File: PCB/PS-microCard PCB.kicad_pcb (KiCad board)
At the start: 4 copper layers, 36.2 x 87.7 mm, 69 parts, among them J1 Oled Socket, J3 MEM2052-00-195-00-A_REVA, J4 10118194-0001LF, J6 JST Debug Connector, SW1 FSM4JSMA, SW2 FSM4JSMA, U1 W25Q128JVS, U2 RP2350_60QFN, U3 TPS2113APWR, U4 TLV75533PDBVR, U5 TPS7A2033PDBVR, Y1 ABM8-272-T3

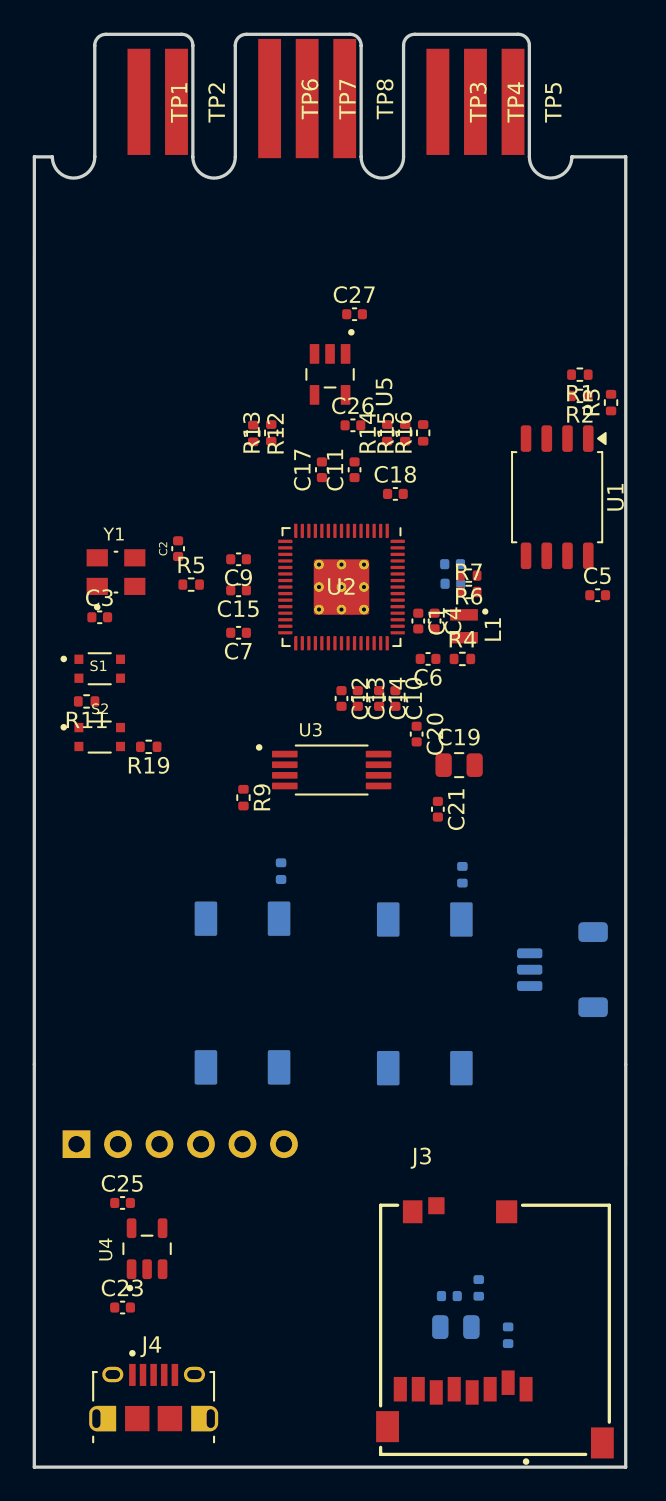
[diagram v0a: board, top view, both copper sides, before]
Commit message: BOM and Gerber files
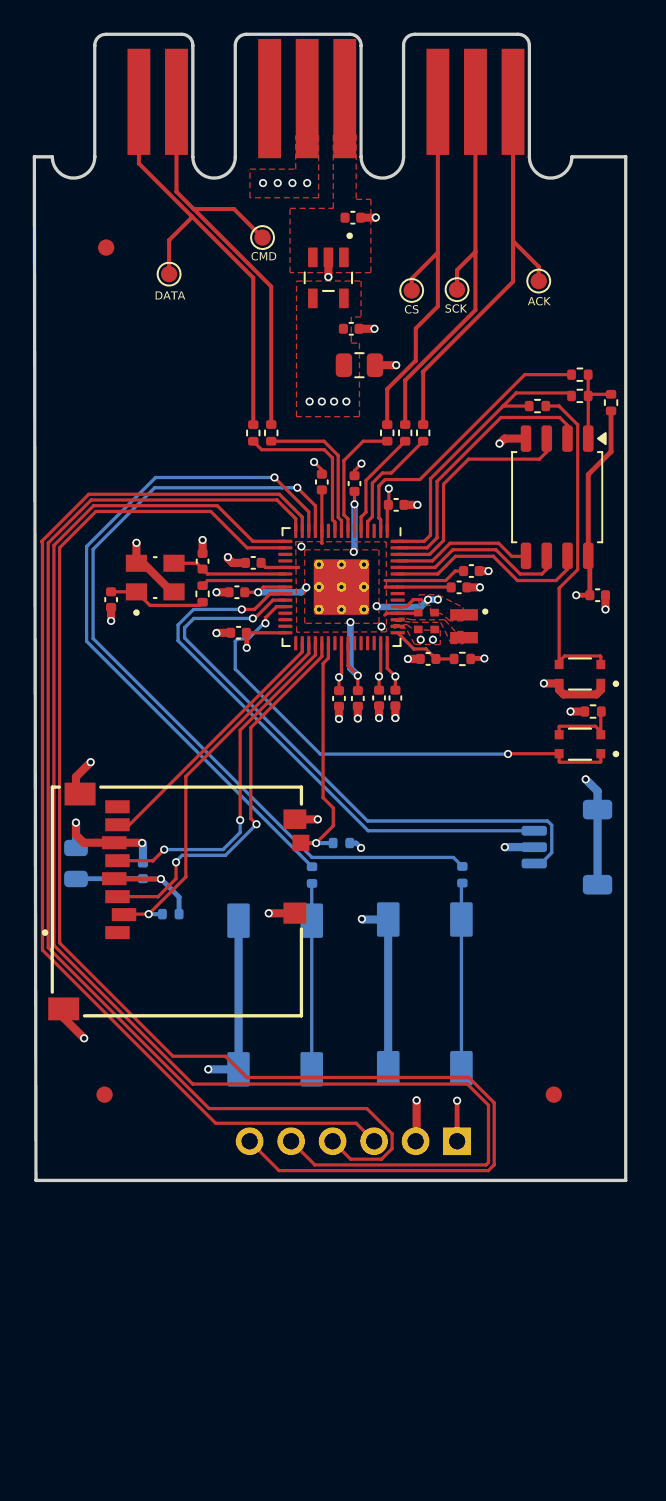
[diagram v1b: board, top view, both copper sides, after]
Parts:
- removed C20, C21: 100n, Capacitor_SMD:C_0402_1005Metric
- removed C23: 1u, Capacitor_SMD:C_0402_1005Metric
- removed C25: 4.7u, Capacitor_SMD:C_0402_1005Metric
- removed J4: 10118194-0001LF, footprints:AMPHENOL_10118194-0001LF
- removed R6, R7: 27, Resistor_SMD:R_0402_1005Metric
- removed R9: 1k, Resistor_SMD:R_0402_1005Metric
- removed U3: TPS2113APWR, footprints:TPS2113-SOP65P640X120-8N
- removed U4: TLV75533PDBVR, footprints:TLV75533PDBVR-SOT95P280X145-5N
- added ?: , , F.Cu at (164.3, 118.5)
- added CMD: PS1_CMD_DBG, TestPoint:TestPoint_Pad_D1.0mm, F.Cu at (146.5, 66.0)
- added DATA: PS1_DATA_DBG, TestPoint:TestPoint_Pad_D1.0mm, F.Cu at (140.8, 68.2)
- added REF**: Fiducial_1mm_Mask3mm, Fiducial:Fiducial_1mm_Mask3mm, F.Cu at (136.8, 118.5)
- added REF**: Fiducial_1mm_Mask3mm, Fiducial:Fiducial_1mm_Mask3mm, F.Cu at (136.9, 66.6)
- added TP11: PS1_CS_DBG, TestPoint:TestPoint_Pad_D1.0mm, F.Cu at (155.6, 69.2)
- added TP12: PS1_SCK_DBG, TestPoint:TestPoint_Pad_D1.0mm, F.Cu at (158.4, 69.2)
- added TP13: PS1_ACK_DBG, TestPoint:TestPoint_Pad_D1.0mm, F.Cu at (163.4, 68.7)
- C1, C4: footprint Capacitor_SMD:C_0402_1005Metric -> footprints:C_0402_1005Metric_small_pads
- C16, C8: moved to F.Cu
- moved C24 36.7 mm to (135.1, 104.3), turned to 90 degrees
- moved R8 33.0 mm to (140.8, 107.4), turned to 0 degrees
- moved J3 32.7 mm to (141.2, 106.6), turned to -90 degrees
- moved C22 32.1 mm to (139.2, 104.8), turned to 90 degrees
- moved R19 31.6 mm to (163.3, 76.3), turned to 0 degrees
- moved R11 31.0 mm to (166.7, 95.0), turned to 0 degrees
- moved S1 29.8 mm to (165.9, 97.0), turned to 180 degrees
- moved S2 29.7 mm to (165.9, 92.7), turned to 180 degrees
- moved R10 28.5 mm to (151.3, 103.0), turned to 180 degrees
- moved C19 25.2 mm to (152.4, 73.8)
- moved J1 23.3 mm to (158.4, 121.3), turned to 90 degrees
- moved J6 7.51 mm to (165.1, 103.3)
- moved C26 5.91 mm to (151.9, 71.6)
- moved C27 5.91 mm to (152.0, 64.8)
- moved U5 5.91 mm to (150.5, 68.5)
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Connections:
- net Net-(U5-EN) renamed /PS1_3V5
- C26 pad 1: /PS1_3V3 -> +3V3
- U2 pad 51: Net-(U2-USB_DM) -> unconnected-(U2-USB_DM-Pad51)
- U2 pad 52: Net-(U2-USB_DP) -> unconnected-(U2-USB_DP-Pad52)
- U5 pad 5: /PS1_3V3 -> +3V3
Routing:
- net /OLED_CS: track 0.00 -> 90.2 mm
- net /OLED_D/C: track 0.00 -> 87.5 mm
- net GND: track 0.00 -> 77.0 mm, vias 0 -> 41
- net /OLED_MOSI: track 0.00 -> 73.3 mm
- net /OLED_SCK: track 0.00 -> 68.8 mm
- net +3V3: track 0.00 -> 58.8 mm, vias 0 -> 16
- net /Left Button: track 0.00 -> 51.0 mm, vias 0 -> 1
- net /Right Button: track 0.00 -> 42.7 mm, vias 0 -> 1
- net /SWD: track 0.00 -> 37.3 mm, vias 0 -> 1
- net /SWCLK: track 0.00 -> 34.9 mm, vias 0 -> 1
- net /RUN: track 0.00 -> 31.4 mm, vias 0 -> 2
- net /PS1_CMD_DBG: track 0.00 -> 27.1 mm
- net /PS1_DATA_DBG: track 0.00 -> 26.8 mm
- net /PS1_ACK_DBG: track 0.00 -> 25.1 mm
- net /PS1_SCK_DBG: track 0.00 -> 24.3 mm
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- added copper zone on F.Cu, net +1V1
- added copper zone on F.Cu, net +3V3
- added copper zone on In2.Cu, net +3V3
- added copper zone on F.Cu, net /PS1_3V5
- added copper zone on F.Cu, net /VREG_LX
- added copper zone on F.Cu, net GND
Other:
- board size 36.2 x 87.7 mm -> 36.2 x 70.2 mm
- board text added: "ACK"
- board text added: "CS"
- board text added: "SCK"
